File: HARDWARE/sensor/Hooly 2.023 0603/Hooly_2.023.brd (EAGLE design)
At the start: 44.2 x 34.5 mm, 36 parts, among them IC2 MCP1703CB, Q1 8MHz Crystal, U3 MCP73831, U5 ATMEGA328P-AU

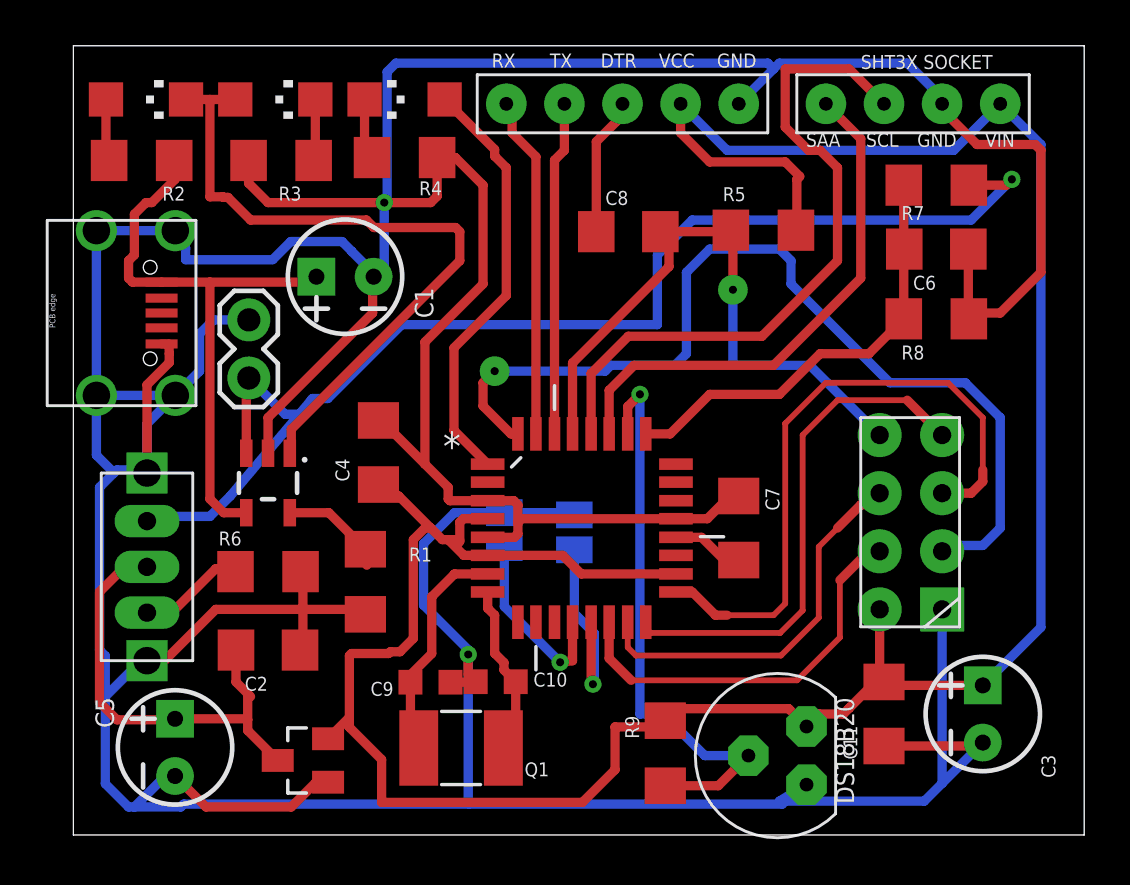
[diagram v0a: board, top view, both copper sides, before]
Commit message: Hardware update
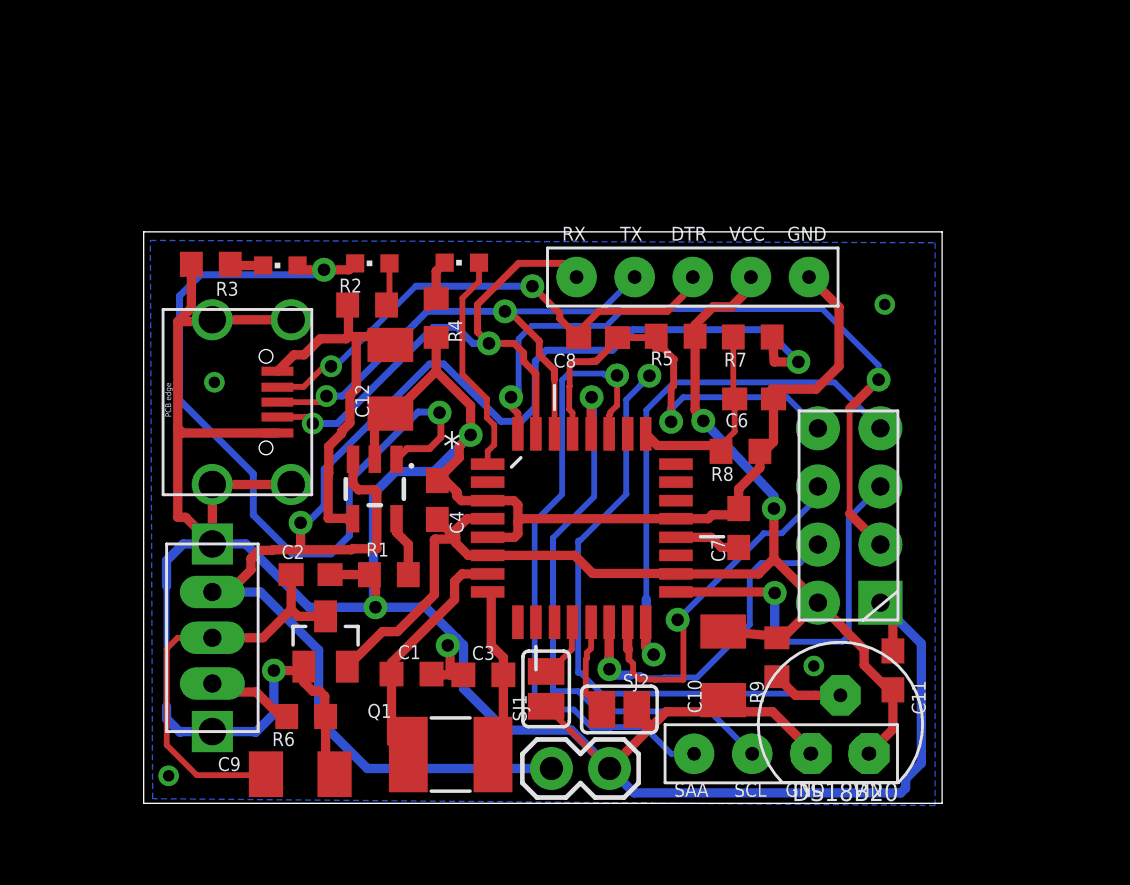
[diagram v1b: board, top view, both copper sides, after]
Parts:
- removed C5: 10uF, SparkFun-Capacitors:CPOL-RADIAL-2.5MM-5MM
- removed U$6: FTDI232, My_library:FTDI232
- added C12: 1uF, resistor:C1206K
- added U$5: FTDI232, My_library:FTDI232
- C1: value 4.7uF -> (none); device SparkFun-Capacitors:CPOL-RADIAL-2.5MM-5MM -> rcl:C0603K
- C10, C9: value 22pF -> 1uF; device rcl:C0603K -> resistor:C1206K
- C11, C2, C4, C6, C7, C8: device resistor:C1206 -> resistor:C0603
- C3: value 10uF -> (none); device SparkFun-Capacitors:CPOL-RADIAL-2.5MM-5MM -> rcl:C0603K
- LED1, LED2, LED4: device led:CHIPLED_1206 -> led:CHIPLED_0603
- Q1: value 8MHz Crystal -> (none)
- R1, R2, R3, R4, R5, R6, R7, R8, R9: device rcl:R1206 -> rcl:R0603
- moved U$1 29.0 mm to (29.0, 1.56)
- moved J2 25.2 mm to (24.1, 0.92), turned to 180 degrees
- moved C3 21.9 mm to (18.6, 5.01), turned to 0 degrees
- moved C1 17.6 mm to (15.4, 5.05), turned to 0 degrees
- moved LED1 12.2 mm to (13.7, 23.0), turned to 90 degrees
- moved R2 11.7 mm to (13.5, 21.2), turned to 0 degrees
- moved R7 10.4 mm to (30.3, 19.8)
- moved R8 10.3 mm to (29.8, 14.8)
- moved C6 10.3 mm to (30.4, 17.1)
- moved C10 9.97 mm to (29.0, 5.41), turned to 270 degrees
- moved SJ2 7.99 mm to (24.5, 3.50), flipped to the top, turned to 0 degrees
- moved LED4 7.56 mm to (17.6, 23.0)
- moved LED2 7.26 mm to (9.68, 22.9), turned to 90 degrees
- moved SJ1 7.18 mm to (21.3, 4.40), flipped to the top
- moved R4 7.14 mm to (16.5, 20.6), turned to 270 degrees
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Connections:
- net DTR: now also U$5.DTR, U$7.D-; no longer U$6.DTR
- net GND: now also C10.2, C12.2, C3.1, SJ1.2, U$5.GND; no longer C10.1, C3.2, C5.2, SJ1.1, U$6.GND
- net N$2: now also C9.1; no longer C5.1
- net RX: now also U$5.TX, U$7.D+; no longer U$6.TX
- net SW1: now also SJ1.1; no longer SJ1.2
- net TX: now also U$5.RX, U$7.ID; no longer U$6.RX
- net VCC: now also C10.1, U$5.VCC; no longer C3.1, U$6.VCC
- net VUSB: now also C12.1; no longer C1.1
- net XTAL1: now also C1.1; no longer C9.1
- net XTAL2: now also C3.2; no longer C10.2
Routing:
- net GND: track 275.4 -> 178.3 mm, vias 2 -> 4
- net VCC: track 121.4 -> 60.2 mm, vias 0 -> 2
- net DTR: track 5.70 -> 22.5 mm, vias 0 -> 2
- net VBATT: track 54.3 -> 66.2 mm, vias 1 -> 2
- net SCK: track 28.1 -> 16.5 mm, vias 0 -> 1
- net CE: track 41.7 -> 30.7 mm, vias 1 -> 2
- net RX: track 14.7 -> 24.9 mm, vias 0 -> 2
- net CKBAT: track 19.2 -> 9.20 mm
- net TX: track 14.6 -> 24.6 mm, vias 0 -> 2
- net RESET: track 29.5 -> 20.0 mm
- net VUSB: track 25.8 -> 16.9 mm
- net N$3: track 18.6 -> 9.80 mm
- net N$8: track 30.7 -> 37.3 mm, vias 0 -> 2
- net SW1: track 8.26 -> 3.39 mm, vias 1 -> 0
- net SCL: track 30.0 -> 25.2 mm, vias 0 -> 1
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- added copper zone on layer 16, net GND
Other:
- board size 44.2 x 34.5 mm -> 34.9 x 25 mm
- board text added: "-"
- board text removed: "GND"
- board text removed: "SHT3X SOCKET"
